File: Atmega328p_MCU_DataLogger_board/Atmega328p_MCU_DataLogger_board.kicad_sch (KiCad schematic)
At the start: 16 parts, among them U1 24LC1025, U2 24LC1025, U3 ATMEGA328P-AU, U4 ds1337s+, Y1 Crystal, Y2 32.768 kHz

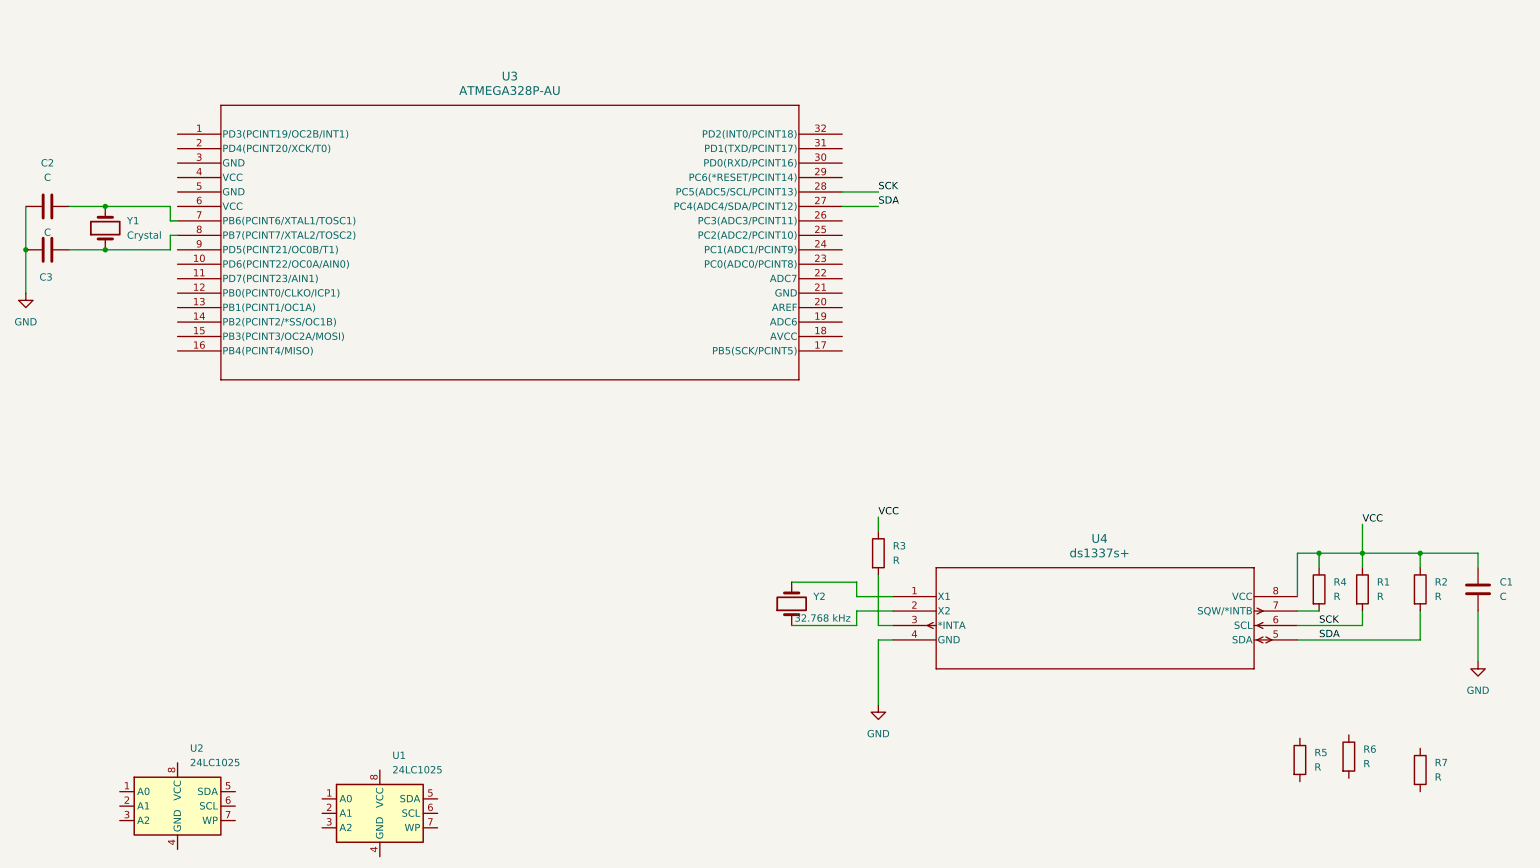
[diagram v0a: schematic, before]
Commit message: MCU DataLogger
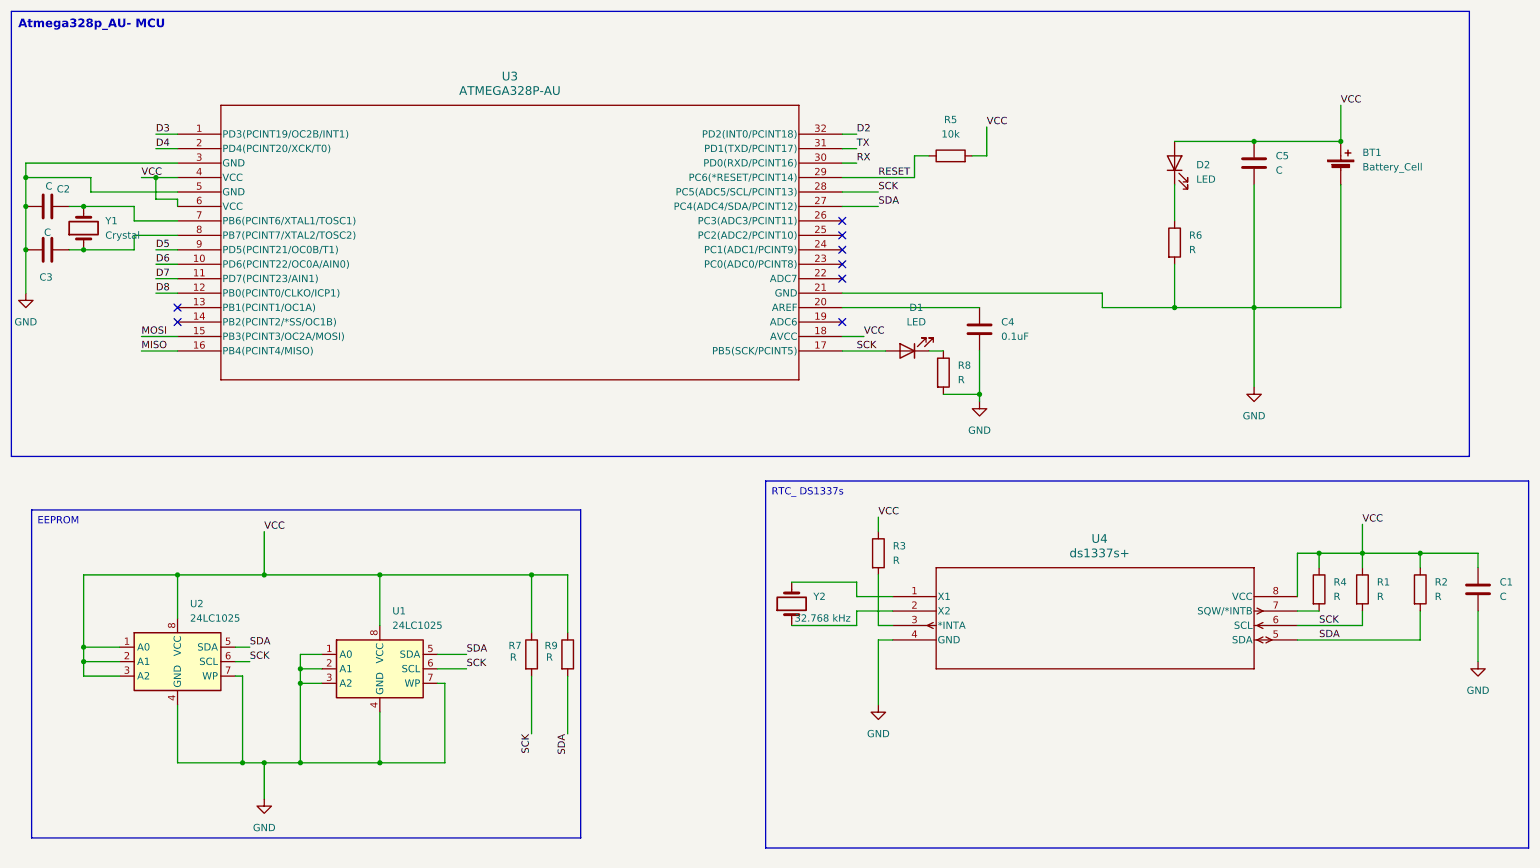
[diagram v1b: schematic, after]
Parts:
- added BT1: Battery_Cell, symbol Device:Battery_Cell
- added C4: 0.1uF, symbol Device:C
- added C5: C, symbol Device:C
- added D1, D2: LED, symbol Device:LED
- added R8, R9: R, symbol Device:R
- R5: value R -> 10k
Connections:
- net GND: now also R6.2, U1.1 (A0), U1.2 (A1), U1.3 (A2), U1.4 (GND), U1.7 (WP), U2.4 (GND), U2.7 (WP), U3.21 (GND), U3.3 (GND), U3.5 (GND), BT1.2 (-), C4.2, C5.2, R8.2
- net SCK: now also R7.2, U1.6 (SCL), U2.6 (SCL), U3.17 (PB5(SCK/PCINT5)), D1.2 (A)
- net SDA: now also U1.5 (SDA), U2.5 (SDA), R9.2
- net VCC: now also R5.2, R7.1, U1.8 (VCC), U2.1 (A0), U2.2 (A1), U2.3 (A2), U2.8 (VCC), U3.18 (AVCC), U3.4 (VCC), U3.6 (VCC), BT1.1 (+), C5.1, D2.2 (A), R9.1
- net RESET: now reaches R5.1
- net RESET: now also U3.29 (PC6(*RESET/PCINT14))
- net at R6.1: now also D2.1 (K)
- net D3: now reaches U3.1 (PD3(PCINT19/OC2B/INT1))
- net D6: now reaches U3.10 (PD6(PCINT22/OC0A/AIN0))
- net D7: now reaches U3.11 (PD7(PCINT23/AIN1))
- net D8: now reaches U3.12 (PB0(PCINT0/CLKO/ICP1))
- net MOSI: now reaches U3.15 (PB3(PCINT3/OC2A/MOSI))
- net MISO: now reaches U3.16 (PB4(PCINT4/MISO))
- net D4: now reaches U3.2 (PD4(PCINT20/XCK/T0))
- net at U3.20 (AREF): now also C4.1
- net RX: now reaches U3.30 (PD0(RXD/PCINT16))
- net TX: now reaches U3.31 (PD1(TXD/PCINT17))
- net D2: now reaches U3.32 (PD2(INT0/PCINT18))
- net D5: now reaches U3.9 (PD5(PCINT21/OC0B/T1))
- new net: D1.1 (K), R8.1
- no-connect marks 0 -> 8
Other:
- title: (none) -> MCU DataLogger
- moved on the sheet: R5, R6, R7, U1, U2, Y1
